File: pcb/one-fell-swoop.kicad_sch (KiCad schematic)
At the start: 20 parts, among them J1 TRRS, SW1 SW_PUSH, SW10 SW_PUSH, SW11 SW_PUSH, SW12 SW_PUSH, SW13 SW_PUSH, SW14 SW_PUSH, SW15 SW_PUSH, SW16 SW_PUSH, SW17 SW_PUSH, SW2 SW_PUSH, SW3 SW_PUSH, SW4 SW_PUSH, SW5 SW_PUSH, SW6 SW_PUSH, SW7 SW_PUSH, SW8 SW_PUSH, SW9 SW_PUSH, U1 ProMicro

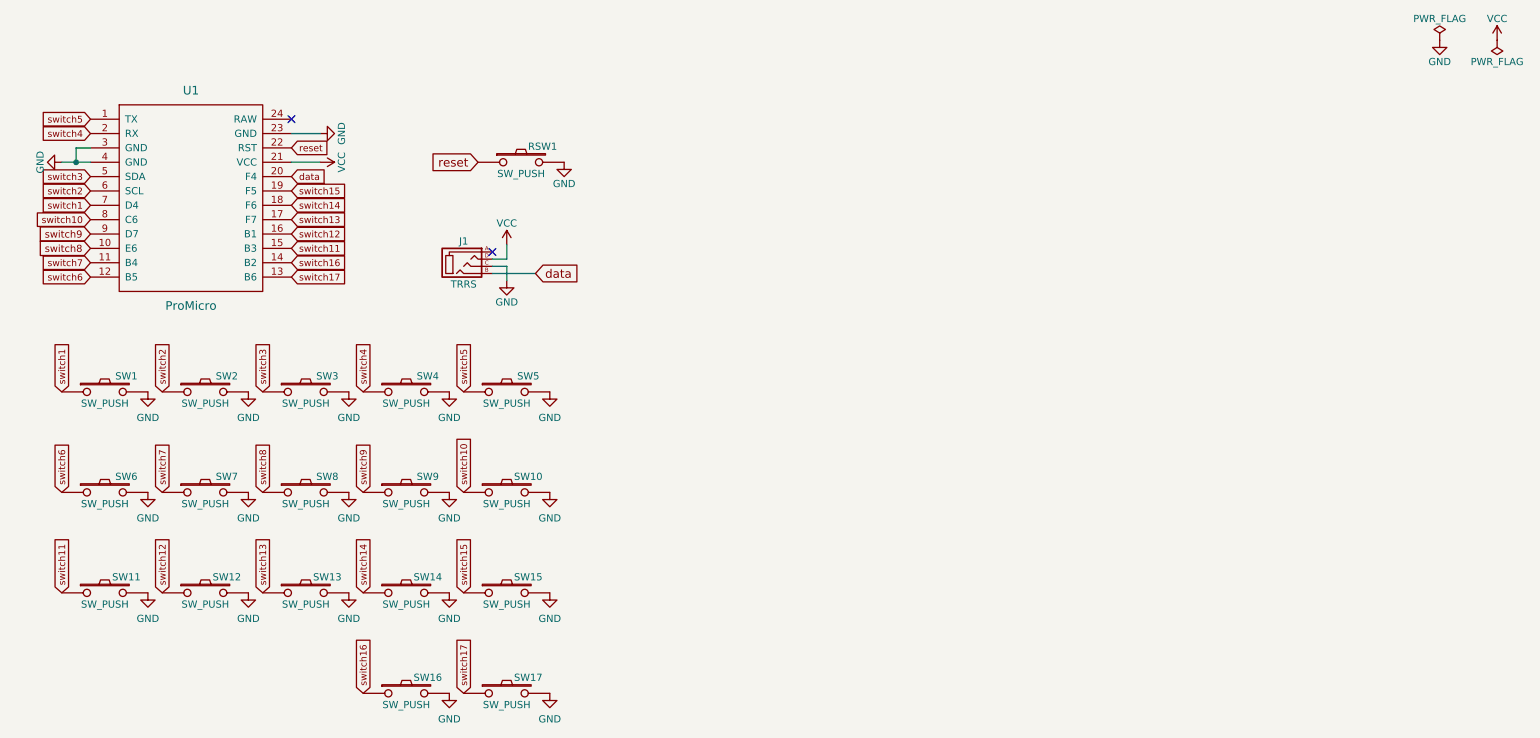
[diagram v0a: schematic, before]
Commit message: Added files for the second version of the Swoop.
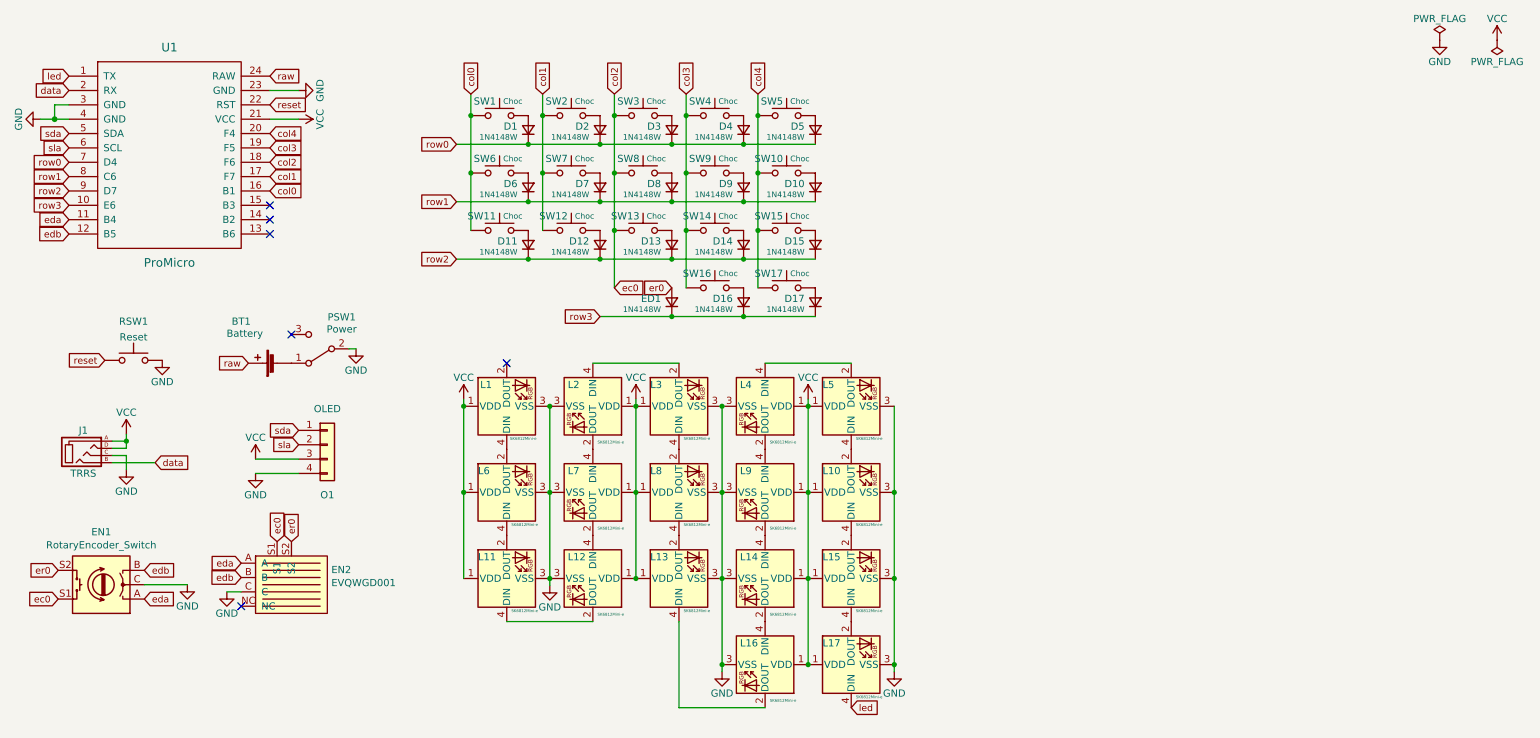
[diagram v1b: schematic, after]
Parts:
- removed RSW1: SW_PUSH, one-fell-swoop:Reset_reversible, symbol one-fell-swoop:SW_PUSH-kbd-corne-light-rescue
- removed SW1, SW10, SW11, SW12, SW13, SW14, SW15, SW16, SW17, SW2, SW3, SW4, SW5, SW6, SW7, SW8, SW9: SW_PUSH, one-fell-swoop:Choc_reversible, symbol one-fell-swoop:SW_PUSH-kbd-corne-light-rescue
- added BT1: Battery, swoop:Battery_pads, symbol Device:Battery_Cell
- added D1, D10, D11, D12, D13, D14, D15, D16, D17, D2, D3, D4, D5, D6, D7, D8, D9, ED1: 1N4148W, swoop:D3_SMD, symbol Device:D_Small
- added EN1: RotaryEncoder_Switch, swoop:RotaryEncoder, symbol Device:RotaryEncoder_Switch
- added EN2: EVQWGD001, swoop:RollerEncoder, symbol swoop:EVQWGD001
- added L1, L10, L11, L12, L13, L14, L15, L16, L17, L2, L3, L4, L5, L6, L7, L8, L9: SK6812Mini-e, swoop:SK6812_Mini_E, symbol swoop:SK6812MINI-E
- added O1: OLED, swoop:OLED_jumpers, symbol Connector_Generic:Conn_01x04
- added PSW1: Power, swoop:Power, symbol Switch:SW_SPDT
- added RSW1: Reset, swoop:Reset, symbol Switch:SW_Push
- added SW1, SW10, SW11, SW12, SW13, SW14, SW15, SW16, SW17, SW2, SW3, SW4, SW5, SW6, SW7, SW8, SW9: Choc, swoop:Choc, symbol Switch:SW_Push
- J1: footprint one-fell-swoop:TRRS_jumpers -> swoop:TRRS-3pin; symbol one-fell-swoop:MJ-4PP-9-kbd-corne-light-rescue -> swoop:MJ-4PP-9-kbd-corne-light-rescue
- U1: footprint one-fell-swoop:ProMicro_jumpers -> swoop:ProMicro_jumpers; symbol one-fell-swoop:ProMicro-kbd-corne-light-rescue -> swoop:ProMicro-kbd-corne-light-rescue
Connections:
- net switch4 is gone; now on net data: U1.2 (RX)
- net GND: now also EN1.C, EN2.C, L1.3 (VSS), L10.3 (VSS), L11.3 (VSS), L12.3 (VSS), L13.3 (VSS), L14.3 (VSS), L15.3 (VSS), L16.3 (VSS), L17.3 (VSS), L2.3 (VSS), L3.3 (VSS), L4.3 (VSS), L5.3 (VSS), L6.3 (VSS), L7.3 (VSS), L8.3 (VSS), L9.3 (VSS), O1.4 (Pin_4), PSW1.2 (B), RSW1.2
- net VCC: now also J1.A, L1.1 (VDD), L10.1 (VDD), L11.1 (VDD), L12.1 (VDD), L13.1 (VDD), L14.1 (VDD), L15.1 (VDD), L16.1 (VDD), L17.1 (VDD), L2.1 (VDD), L3.1 (VDD), L4.1 (VDD), L5.1 (VDD), L6.1 (VDD), L7.1 (VDD), L8.1 (VDD), L9.1 (VDD), O1.3 (Pin_3)
- net data: no longer U1.20 (F4)
- net reset: now also RSW1.1
- net raw: now reaches U1.24 (RAW)
- net raw: now also BT1.1 (+)
- net switch1 renamed row0
- net row0: now also D1.1 (K), D2.1 (K), D3.1 (K), D4.1 (K), D5.1 (K)
- net switch10 renamed row1
- net row1: now also D10.1 (K), D6.1 (K), D7.1 (K), D8.1 (K), D9.1 (K)
- net switch11: no longer names the net of U1.15 (B3)
- net switch12 renamed col0
- net col0: now also SW1.1, SW11.1, SW6.1
- net switch13 renamed col1
- net col1: now also SW12.1, SW2.1, SW7.1
- net switch14 renamed col2
- net col2: now also EN1.S1, EN2.S1, SW13.1, SW3.1, SW8.1
- net switch15 renamed col3
- net col3: now also SW14.1, SW16.1, SW4.1, SW9.1
- net switch16: no longer names the net of U1.14 (B2)
- net switch17: no longer names the net of U1.13 (B6)
- net switch2 renamed sla
- net sla: now also O1.2 (Pin_2)
- net switch3 renamed sda
- net sda: now also O1.1 (Pin_1)
- net switch5 renamed led
- net led: now also L17.4 (DIN)
- net switch6 renamed edb
- net edb: now also EN1.B, EN2.B
- net switch7 renamed eda
- net eda: now also EN1.A, EN2.A
- net switch8 renamed row3
- net row3: now also D16.1 (K), D17.1 (K), ED1.1 (K)
- net switch9 renamed row2
- net row2: now also D11.1 (K), D12.1 (K), D13.1 (K), D14.1 (K), D15.1 (K)
- new net: D4.2 (A), SW4.2
- new net: L10.4 (DIN), L15.2 (DOUT)
- new net: L15.4 (DIN), L17.2 (DOUT)
- new net: D11.2 (A), SW11.2
- new net: D2.2 (A), SW2.2
- new net: D3.2 (A), SW3.2
- new net: L1.4 (DIN), L6.2 (DOUT)
- new net: L11.2 (DOUT), L6.4 (DIN)
- new net: L13.2 (DOUT), L8.4 (DIN)
- new net: L13.4 (DIN), L16.2 (DOUT)
- new net: D6.2 (A), SW6.2
- new net: D10.2 (A), SW10.2
- new net: D8.2 (A), SW8.2
- new net: L14.4 (DIN), L9.2 (DOUT)
- new net: L4.2 (DOUT), L9.4 (DIN)
- new net: D9.2 (A), SW9.2
- new net: D1.2 (A), SW1.2
- new net: L4.4 (DIN), L5.2 (DOUT)
- new net: L10.2 (DOUT), L5.4 (DIN)
- new net: BT1.2 (-), PSW1.1 (A)
- new net: D13.2 (A), SW13.2
- new net: D17.2 (A), SW17.2
- new net: L12.4 (DIN), L7.2 (DOUT)
- new net: L2.2 (DOUT), L7.4 (DIN)
- new net: L2.4 (DIN), L3.2 (DOUT)
- new net: L11.4 (DIN), L12.2 (DOUT)
- new net: D5.2 (A), SW5.2
- new net: D12.2 (A), SW12.2
- new net: D7.2 (A), SW7.2
- new net: D16.2 (A), SW16.2
- new net: L14.2 (DOUT), L16.4 (DIN)
- new net: L3.4 (DIN), L8.2 (DOUT)
- new net: D15.2 (A), SW15.2
- new net: D14.2 (A), SW14.2
- new net col4: SW10.1, SW15.1, SW17.1, SW5.1, U1.20 (F4)
- new net er0: ED1.2 (A), EN1.S2, EN2.S2
- no-connect marks 2 -> 6
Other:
- moved on the sheet: J1, U1
